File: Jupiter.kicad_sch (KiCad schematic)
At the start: 341 parts, among them J1 Conn_01x04, SW1 SW_Push, U1 ATmega32U4-M, Y1 Crystal_GND24_Small

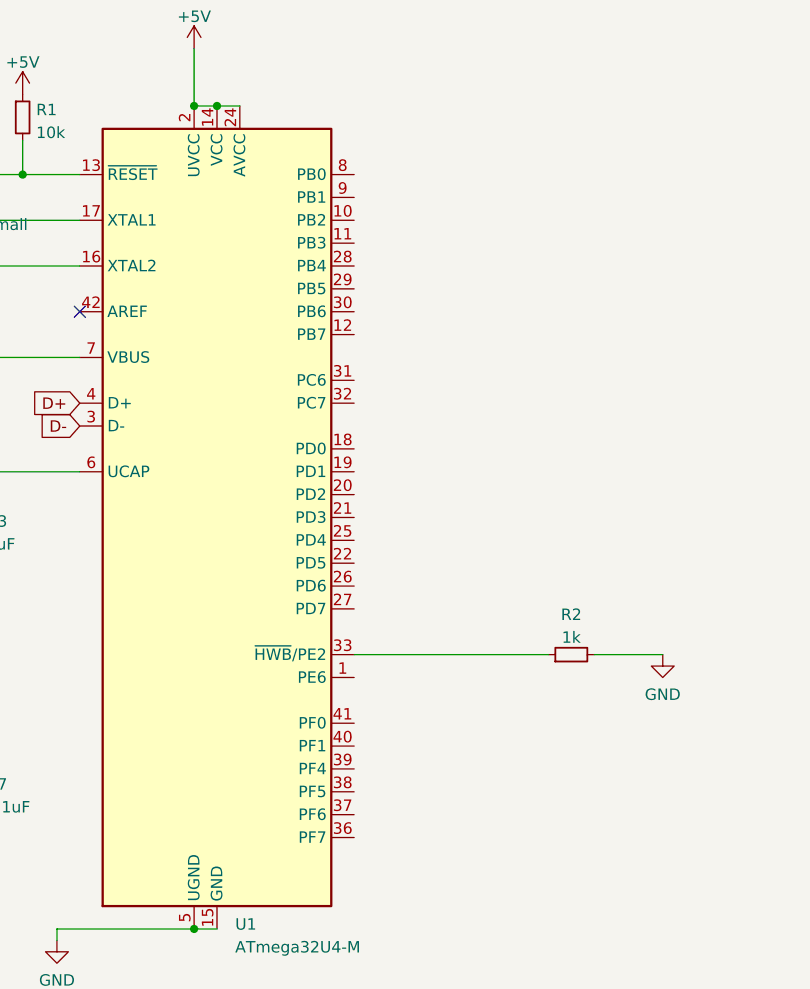
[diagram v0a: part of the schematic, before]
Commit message: Placed keys on board
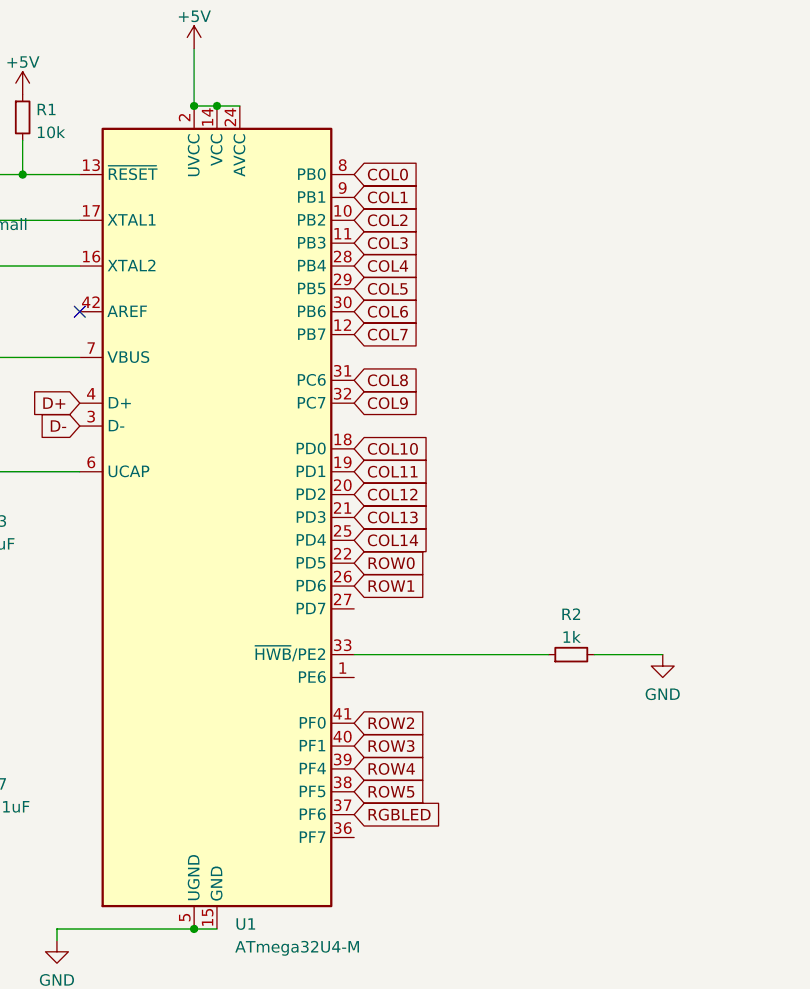
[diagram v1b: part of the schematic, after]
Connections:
- net COL0: now also U1.8 (PB0)
- net COL1: now also U1.9 (PB1)
- net COL10: now also U1.18 (PD0)
- net COL11: now also U1.19 (PD1)
- net COL12: now also U1.20 (PD2)
- net COL13: now also U1.21 (PD3)
- net COL14: now also U1.25 (PD4)
- net COL2: now also U1.10 (PB2)
- net COL3: now also U1.11 (PB3)
- net COL4: now also U1.28 (PB4)
- net COL5: now also U1.29 (PB5)
- net COL6: now also U1.30 (PB6)
- net COL7: now also U1.12 (PB7)
- net COL8: now also U1.31 (PC6)
- net COL9: now also U1.32 (PC7)
- net RGBLED: now also U1.37 (PF6)
- net ROW0: now also U1.22 (PD5)
- net ROW1: now also U1.26 (PD6)
- net ROW2: now also U1.41 (PF0)
- net ROW3: now also U1.40 (PF1)
- net ROW4: now also U1.39 (PF4)
- net ROW5: now also U1.38 (PF5)
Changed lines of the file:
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@@
+    )
+  )
+  (global_label "COL1" (shape input) (at 391.16 36.83 0) (fields_autoplaced)
+    (effects (font (size 1.27 1.27)) (justify left))
+    (property "Intersheet References" "${INTERSHEET_REFS}" (id 0) (at 398.4112 36.7506 0)
+      (effects (font (size 1.27 1.27)) (justify left) hide)
     )
   )
@@
     )
   )
+  (global_label "COL0" (shape input) (at 391.16 34.29 0) (fields_autoplaced)
+    (effects (font (size 1.27 1.27)) (justify left))
+    (property "Intersheet References" "${INTERSHEET_REFS}" (id 0) (at 398.4112 34.2106 0)
+      (effects (font (size 1.27 1.27)) (justify left) hide)
+    )
+  )
   (global_label "ROW3" (shape input) (at 29.21 95.25 180) (fields_autoplaced)
     (effects (font (size 1.27 1.27)) (justify right))
@@
     )
   )
+  (global_label "COL3" (shape input) (at 391.16 41.91 0) (fields_autoplaced)
+    (effects (font (size 1.27 1.27)) (justify left))
+    (property "Intersheet References" "${INTERSHEET_REFS}" (id 0) (at 398.4112 41.8306 0)
+      (effects (font (size 1.27 1.27)) (justify left) hide)
+    )
+  )
+  (global_label "ROW3" (shape input) (at 391.16 97.79 0) (fields_autoplaced)
+    (effects (font (size 1.27 1.27)) (justify left))
+    (property "Intersheet References" "${INTERSHEET_REFS}" (id 0) (at 398.8345 97.8694 0)
+      (effects (font (size 1.27 1.27)) (justify left) hide)
+    )
+  )
+  (global_label "ROW1" (shape input) (at 391.16 80.01 0) (fields_autoplaced)
+    (effects (font (size 1.27 1.27)) (justify left))
+    (property "Intersheet References" "${INTERSHEET_REFS}" (id 0) (at 398.8345 80.0894 0)
+      (effects (font (size 1.27 1.27)) (justify left) hide)
+    )
+  )
+  (global_label "COL13" (shape input) (at 391.16 72.39 0) (fields_autoplaced)
+    (effects (font (size 1.27 1.27)) (justify left))
+    (property "Intersheet References" "${INTERSHEET_REFS}" (id 0) (at 399.6207 72.3106 0)
+      (effects (font (size 1.27 1.27)) (justify left) hide)
+    )
+  )
   (global_label "COL9" (shape input) (at 195.58 21.59 90) (fields_autoplaced)
     (effects (font (size 1.27 1.27)) (justify left))
@@
     )
   )
+  (global_label "COL6" (shape input) (at 391.16 49.53 0) (fields_autoplaced)
+    (effects (font (size 1.27 1.27)) (justify left))
+    (property "Intersheet References" "${INTERSHEET_REFS}" (id 0) (at 398.4112 49.4506 0)
+      (effects (font (size 1.27 1.27)) (justify left) hide)
+    )
+  )
+  (global_label "COL11" (shape input) (at 391.16 67.31 0) (fields_autoplaced)
+    (effects (font (size 1.27 1.27)) (justify left))
+    (property "Intersheet References" "${INTERSHEET_REFS}" (id 0) (at 399.6207 67.2306 0)
+      (effects (font (size 1.27 1.27)) (justify left) hide)
+    )
+  )
+  (global_label "COL10" (shape input) (at 391.16 64.77 0) (fields_autoplaced)
+    (effects (font (size 1.27 1.27)) (justify left))
+    (property "Intersheet References" "${INTERSHEET_REFS}" (id 0) (at 399.6207 64.6906 0)
+      (effects (font (size 1.27 1.27)) (justify left) hide)
+    )
+  )
   (global_label "COL6" (shape input) (at 146.05 21.59 90) (fields_autoplaced)
     (effects (font (size 1.27 1.27)) (justify left))
@@
     )
   )
+  (global_label "COL2" (shape input) (at 391.16 39.37 0) (fields_autoplaced)
+    (effects (font (size 1.27 1.27)) (justify left))
+    (property "Intersheet References" "${INTERSHEET_REFS}" (id 0) (at 398.4112 39.2906 0)
+      (effects (font (size 1.27 1.27)) (justify left) hide)
+    )
+  )
+  (global_label "ROW5" (shape input) (at 391.16 102.87 0) (fields_autoplaced)
+    (effects (font (size 1.27 1.27)) (justify left))
+    (property "Intersheet References" "${INTERSHEET_REFS}" (id 0) (at 398.8345 102.9494 0)
+      (effects (font (size 1.27 1.27)) (justify left) hide)
+    )
+  )
   (global_label "COL5" (shape input) (at 128.27 21.59 90) (fields_autoplaced)
     (effects (font (size 1.27 1.27)) (justify left))
@@
     )
   )
+  (global_label "ROW0" (shape input) (at 391.16 77.47 0) (fields_autoplaced)
+    (effects (font (size 1.27 1.27)) (justify left))
+    (property "Intersheet References" "${INTERSHEET_REFS}" (id 0) (at 398.8345 77.5494 0)
+      (effects (font (size 1.27 1.27)) (justify left) hide)
+    )
+  )
   (global_label "D-" (shape input) (at 360.68 62.23 180) (fields_autoplaced)
     (effects (font (size 1.27 1.27)) (justify right))
@@
     )
   )
+  (global_label "ROW4" (shape input) (at 391.16 100.33 0) (fields_autoplaced)
+    (effects (font (size 1.27 1.27)) (justify left))
+    (property "Intersheet References" "${INTERSHEET_REFS}" (id 0) (at 398.8345 100.4094 0)
+      (effects (font (size 1.27 1.27)) (justify left) hide)
+    )
+  )
+  (global_label "RGBLED" (shape input) (at 391.16 105.41 0) (fields_autoplaced)
+    (effects (font (size 1.27 1.27)) (justify left))
+    (property "Intersheet References" "${INTERSHEET_REFS}" (id 0) (at 400.8302 105.4894 0)
+      (effects (font (size 1.27 1.27)) (justify left) hide)
+    )
+  )
+  (global_label "COL8" (shape input) (at 391.16 57.15 0) (fields_autoplaced)
+    (effects (font (size 1.27 1.27)) (justify left))
+    (property "Intersheet References" "${INTERSHEET_REFS}" (id 0) (at 398.4112 57.0706 0)
+      (effects (font (size 1.27 1.27)) (justify left) hide)
+    )
+  )
+  (global_label "COL4" (shape input) (at 391.16 44.45 0) (fields_autoplaced)
+    (effects (font (size 1.27 1.27)) (justify left))
+    (property "Intersheet References" "${INTERSHEET_REFS}" (id 0) (at 398.4112 44.3706 0)
+      (effects (font (size 1.27 1.27)) (justify left) hide)
+    )
+  )
   (global_label "COL7" (shape input) (at 162.56 21.59 90) (fields_autoplaced)
     (effects (font (size 1.27 1.27)) (justify left))
@@
     )
   )
+  (global_label "COL7" (shape input) (at 391.16 52.07 0) (fields_autoplaced)
+    (effects (font (size 1.27 1.27)) (justify left))
+    (property "Intersheet References" "${INTERSHEET_REFS}" (id 0) (at 398.4112 51.9906 0)
+      (effects (font (size 1.27 1.27)) (justify left) hide)
+    )
+  )
+  (global_label "COL9" (shape input) (at 391.16 59.69 0) (fields_autoplaced)
+    (effects (font (size 1.27 1.27)) (justify left))
+    (property "Intersheet References" "${INTERSHEET_REFS}" (id 0) (at 398.4112 59.6106 0)
+      (effects (font (size 1.27 1.27)) (justify left) hide)
+    )
+  )
   (global_label "ROW1" (shape input) (at 29.21 57.15 180) (fields_autoplaced)
     (effects (font (size 1.27 1.27)) (justify right))
@@
     )
   )
+  (global_label "ROW2" (shape input) (at 391.16 95.25 0) (fields_autoplaced)
+    (effects (font (size 1.27 1.27)) (justify left))
+    (property "Intersheet References" "${INTERSHEET_REFS}" (id 0) (at 398.8345 95.3294 0)
+      (effects (font (size 1.27 1.27)) (justify left) hide)
+    )
+  )
   (global_label "ROW5" (shape input) (at 29.21 133.35 180) (fields_autoplaced)
     (effects (font (size 1.27 1.27)) (justify right))
@@
     )
   )
+  (global_label "COL5" (shape input) (at 391.16 46.99 0) (fields_autoplaced)
+    (effects (font (size 1.27 1.27)) (justify left))
+    (property "Intersheet References" "${INTERSHEET_REFS}" (id 0) (at 398.4112 46.9106 0)
+      (effects (font (size 1.27 1.27)) (justify left) hide)
+    )
+  )
   (global_label "COL4" (shape input) (at 111.76 21.59 90) (fields_autoplaced)
     (effects (font (size 1.27 1.27)) (justify left))
@@
       (effects (font (size 1.27 1.27)) (justify left) hide)
     )
+  )
+  (global_label "COL12" (shape input) (at 391.16 69.85 0) (fields_autoplaced)
+    (effects (font (size 1.27 1.27)) (justify left))
+    (property "Intersheet References" "${INTERSHEET_REFS}" (id 0) (at 399.6207 69.7706 0)
+      (effects (font (size 1.27 1.27)) (justify left) hide)
+    )
+  )
+  (global_label "COL14" (shape input) (at 391.16 74.93 0) (fields_autoplaced)
+    (effects (font (size 1.27 1.27)) (justify left))
+    (property "Intersheet References" "${INTERSHEET_REFS}" (id 0) (at 399.6207 74.8506 0)
+      (effects (font (size 1.27 1.27)) (justify left) hide)
+    )
